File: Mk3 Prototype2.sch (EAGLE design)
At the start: 142 parts, among them IC1 TPD3E001DRL, IC2 TPS62082, IC3 STM32F401V, IC4 BQ2409X, IC40 MCP73831, IC6 CC3100MOD, IC7 BQ2970, J1 ZX62-AB-5PA(11), J2 ER-TFT024-3, J3 SWD_SHROUD, Q1 DMMT5401, Q2 CSD25402Q3A, Q3 CSD13202Q2, Q4 CSD85301Q2, Q6 CSD25402Q3A, Q8 CSD13202Q2, SW1 JOYSTICK_MINI_MULTICOMP, U4 USD-SOCKETNEW, X2 16MHz-3.2-2.5, X3 ABS07-32.768KHZ-T

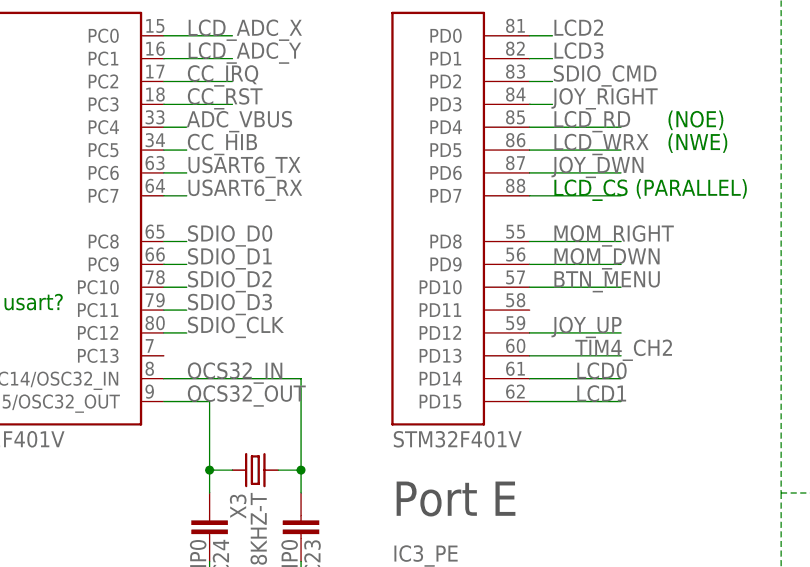
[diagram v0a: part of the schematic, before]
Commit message: load more routing
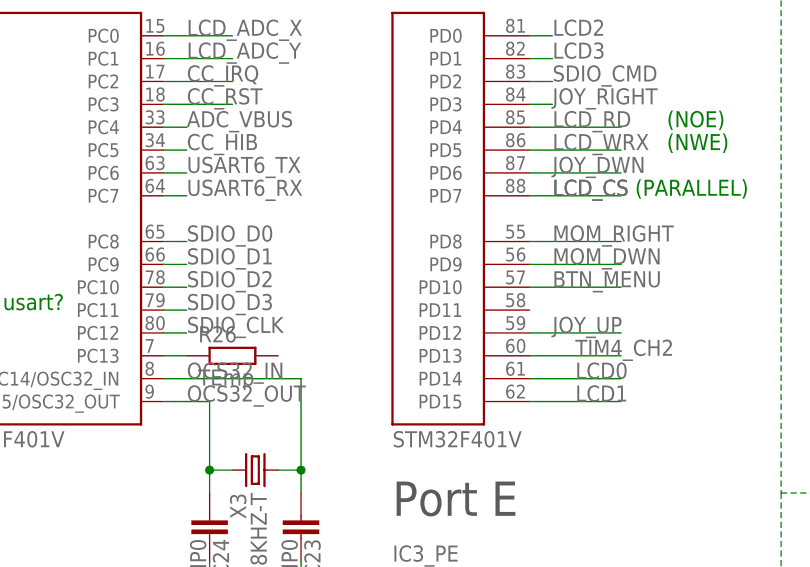
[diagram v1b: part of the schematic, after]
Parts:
- added R26: TEmp, TiLDA Mk3 Parts:R-EU_0603K-SMALL
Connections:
- new net N$8: IC3_PC.PC13, R26.1
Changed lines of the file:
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@@
 <part name="GND14" library="TiLDA Mk3 Parts" deviceset="GND" device=""/>
 <part name="R24" library="TiLDA Mk3 Parts" deviceset="R-EU_" device="0603K-SMALL" value="0/dnp"/>
+<part name="R26" library="TiLDA Mk3 Parts" deviceset="R-EU_" device="0603K-SMALL" value="TEmp"/>
 </parts>
 <sheets>
@@
 <instance part="GND14" gate="1" x="581.66" y="-20.32"/>
 <instance part="R24" gate="G$1" x="332.74" y="299.72" rot="R180"/>
+<instance part="R26" gate="G$1" x="40.64" y="99.06"/>
 </instances>
 <busses>
@@
 <pinref part="IC3" gate="_PD" pin="PD7"/>
 <wire x1="73.66" y1="116.84" x2="83.82" y2="116.84" width="0.1524" layer="91"/>
+<label x="76.2" y="116.84" size="1.778" layer="95"/>
 </segment>
 <segment>
@@
 </segment>
 </net>
+<net name="N$8" class="0">
+<segment>
+<pinref part="IC3" gate="_PC" pin="PC13"/>
+<pinref part="R26" gate="G$1" pin="1"/>
+<wire x1="33.02" y1="99.06" x2="35.56" y2="99.06" width="0.1524" layer="91"/>
+</segment>
+</net>
